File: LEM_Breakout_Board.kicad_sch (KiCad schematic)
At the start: 5 parts, among them J1 Conn_01x06_Male, J2 Conn_01x04_Female

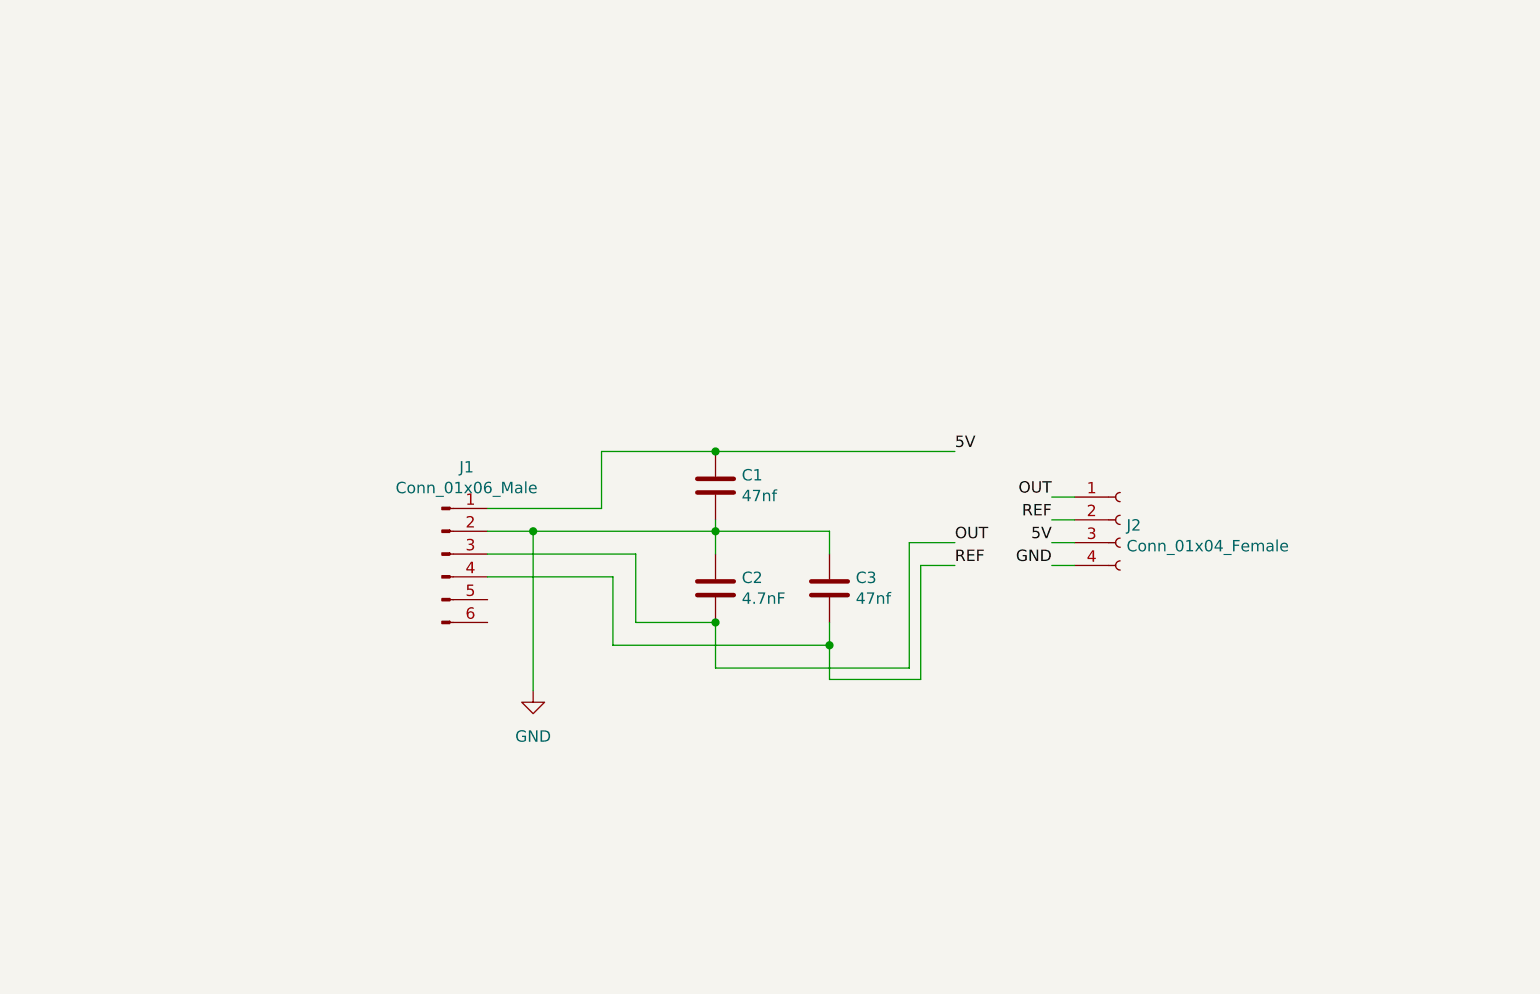
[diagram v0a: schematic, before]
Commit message: Started Redesign
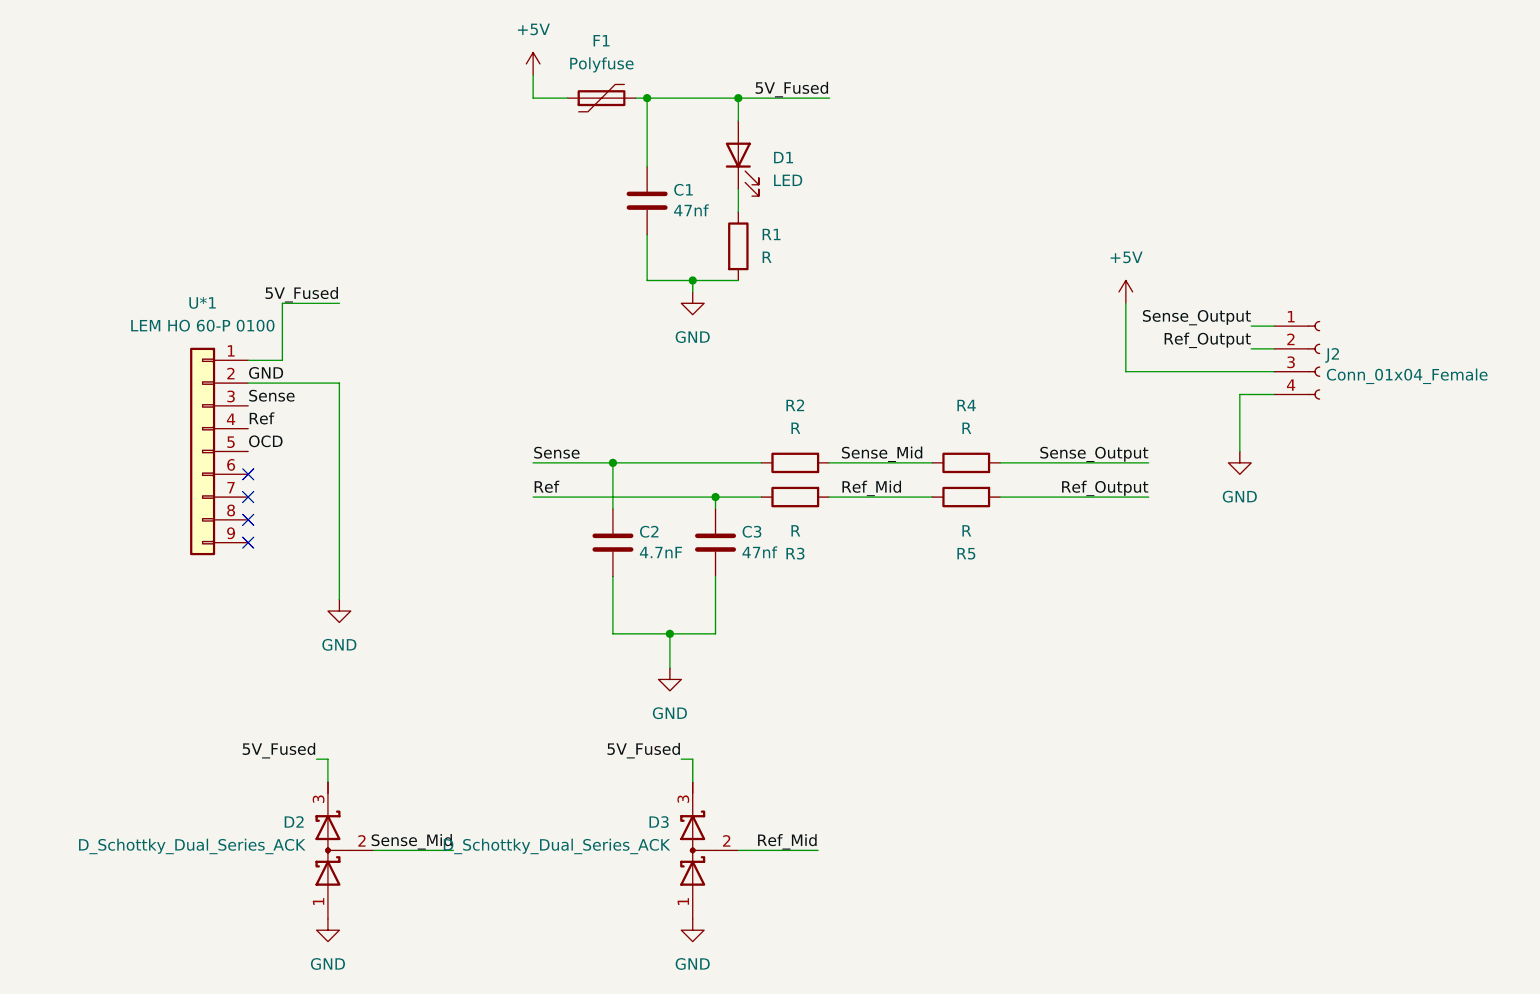
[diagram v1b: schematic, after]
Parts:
- removed J1: Conn_01x06_Male, user:LEM_HAIS_50-P, symbol Connector:Conn_01x06_Male
- added D1: LED, LED_SMD:LED_0603_1608Metric, symbol Device:LED
- added D2, D3: D_Schottky_Dual_Series_ACK, Package_TO_SOT_SMD:SOT-23, symbol Device:D_Schottky_Dual_Series_ACK
- added F1: Polyfuse, Fuse:Fuse_0603_1608Metric, symbol Device:Polyfuse
- added R1, R2, R3, R4, R5: R, Resistor_SMD:R_0603_1608Metric, symbol Device:R
- added U*1: LEM HO 60-P 0100, Sensor_Current:LEM_HO40-NP, symbol Connector_Generic:Conn_01x09
- C1, C2, C3: footprint Capacitor_THT:C_Disc_D3.4mm_W2.1mm_P2.50mm -> Capacitor_SMD:C_0603_1608Metric
- J2: footprint Connector_PinHeader_2.00mm:PinHeader_1x04_P2.00mm_Vertical -> Connector_JST:JST_PH_S4B-PH-SM4-TB_1x04-1MP_P2.00mm_Horizontal
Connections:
- net GND: now also C2.2, C3.2, D2.1 (A), D3.1 (A), R1.2, U*1.2 (Pin_2); no longer C2.1, C3.1
- net 5V renamed +5V
- net +5V: now also F1.1; no longer C1.1
- net OUT renamed Sense_Output
- net Sense_Output: now also R4.2; no longer C2.2
- net REF renamed Ref_Output
- net Ref_Output: now also R5.2; no longer C3.2
- new net: D1.1 (K), R1.1
- new net 5V_Fused: C1.1, D1.2 (A), D2.3 (K), D3.3 (K), F1.2, U*1.1 (Pin_1)
- new net OCD: U*1.5 (Pin_5)
- new net Ref: C3.1, R3.1, U*1.4 (Pin_4)
- new net Ref_Mid: D3.2 (common), R3.2, R5.1
- new net Sense: C2.1, R2.1, U*1.3 (Pin_3)
- new net Sense_Mid: D2.2 (common), R2.2, R4.1
- no-connect marks 0 -> 4
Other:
- moved on the sheet: C1, C2, C3, J2
